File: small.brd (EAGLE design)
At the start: 19 x 30.1 mm, 4 parts, among them U1 SN74LS241N

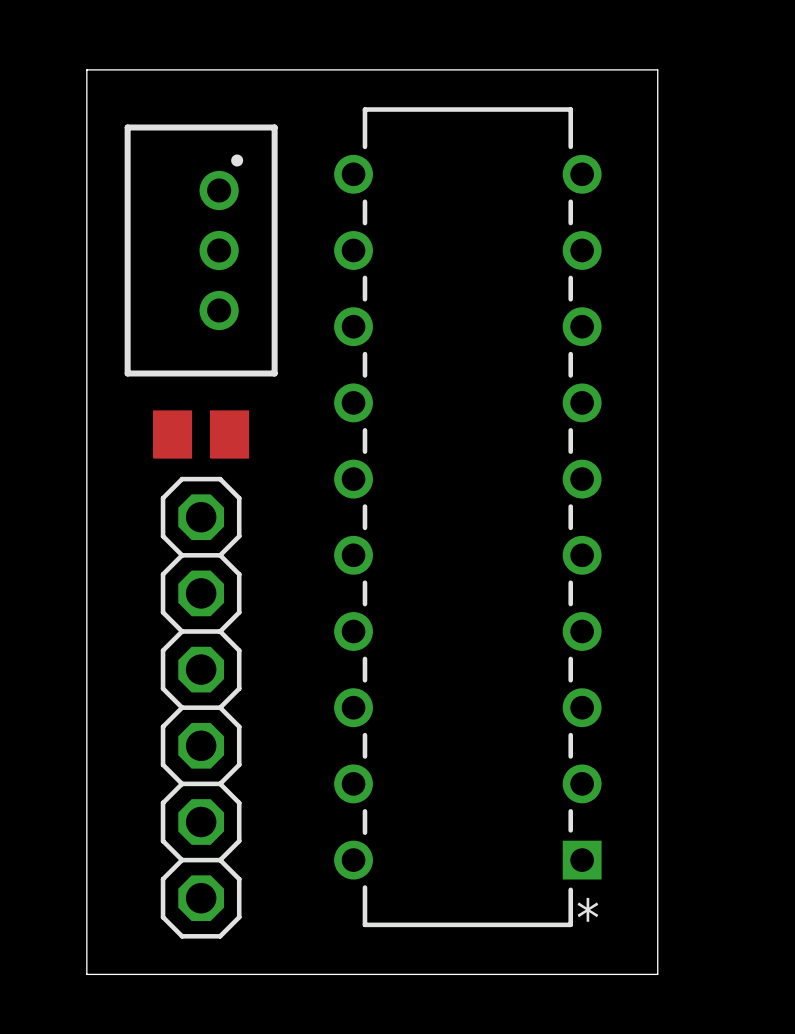
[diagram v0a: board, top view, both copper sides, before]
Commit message: Add files via upload
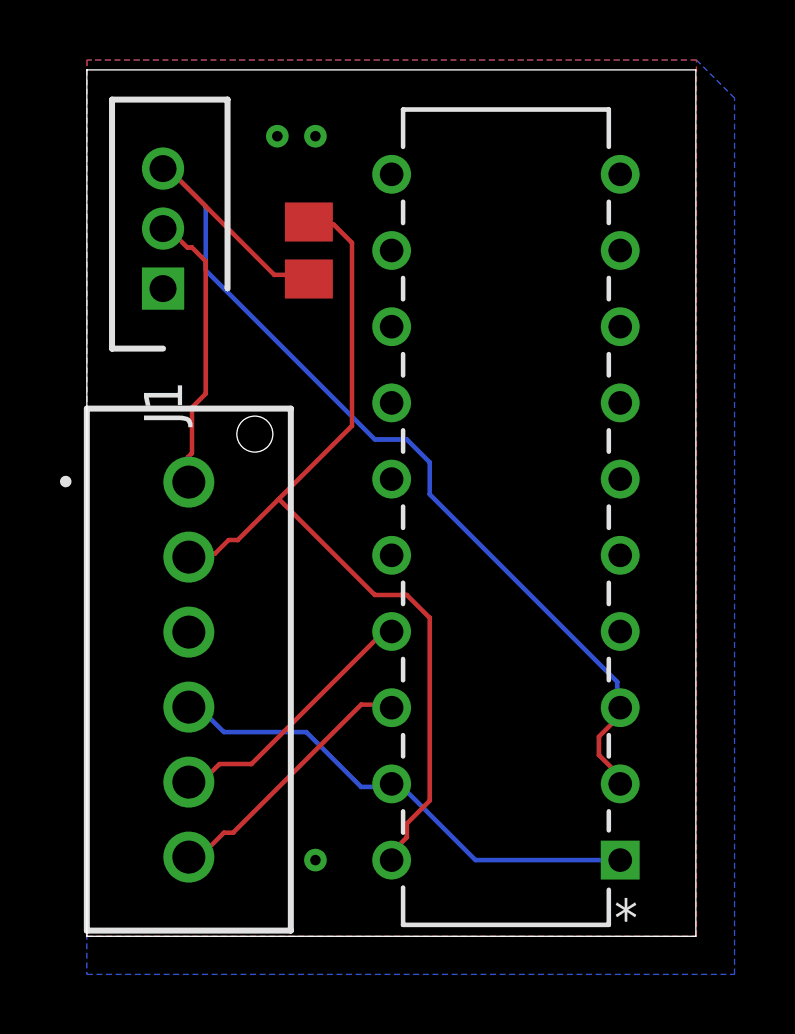
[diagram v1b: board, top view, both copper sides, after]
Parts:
- removed JP1: (no value), adafruit:1X06
- added J2: 53375-0610, wire to board_molex:53375-0610
- J1: value (none) -> 53253-0370; device Wurth_Connectors_WR-WTB:62000311622 -> xl320_molex:SHDR3W50P0X200_1X3_800X365X570
- moved R1 7.10 mm to (7.40, 24.1), turned to 270 degrees
- moved J1 1.80 mm to (2.54, 22.9)
- moved U1 1.27 mm to (10.2, 26.7)
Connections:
- net 5V: now also J2.2; no longer JP1.2
- net 7.4V: now also J2.1; no longer JP1.1
- net DATA_CONTROL: now also J2.4; no longer JP1.4
- net GND: now also J2.3; no longer JP1.3
- net RX: now also J2.6; no longer JP1.6
- net TX: now also J2.5; no longer JP1.5
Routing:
- net DATA: track 0.00 -> 34.8 mm
- net 5V: track 0.00 -> 30.4 mm
- net DATA_CONTROL: track 0.00 -> 16.6 mm
- net 7.4V: track 0.00 -> 9.50 mm
- net RX: track 0.00 -> 8.90 mm
- net TX: track 0.00 -> 8.85 mm
- added copper zone on layer 1, net GND
- added copper zone on layer 16, net GND
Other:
- board size 19 x 30.1 mm -> 20.3 x 28.9 mm
